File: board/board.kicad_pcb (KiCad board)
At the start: 2 copper layers, 21 x 13 mm, 1 part

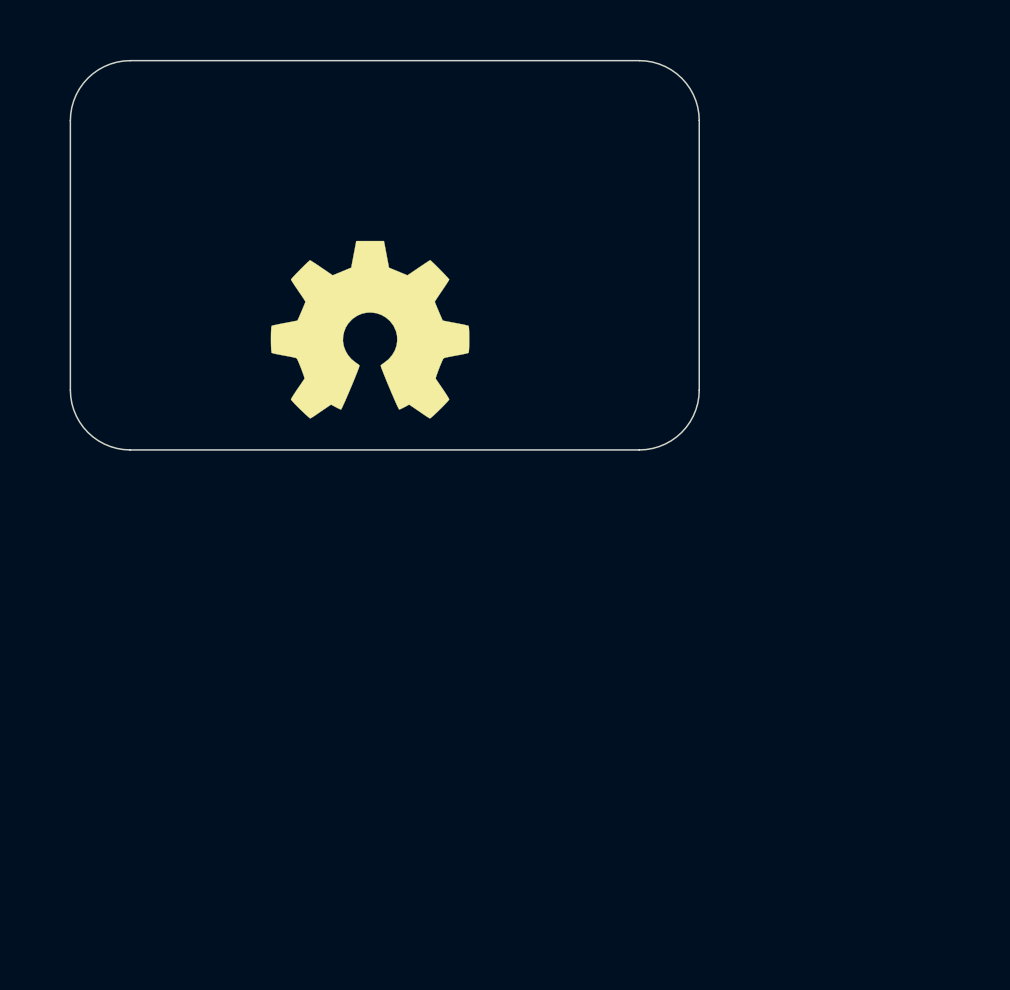
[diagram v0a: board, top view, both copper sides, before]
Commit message: initial
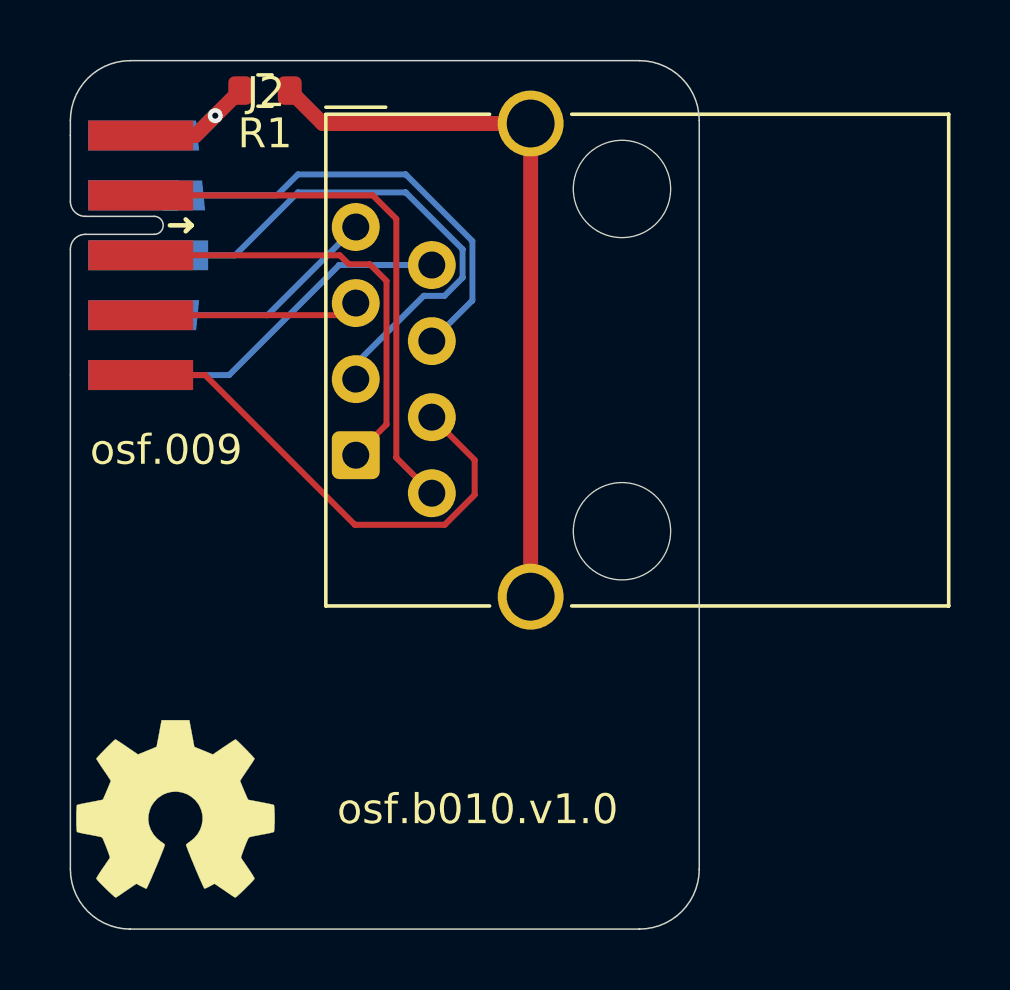
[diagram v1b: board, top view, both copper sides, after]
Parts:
- added J1: 009_1000BASE-T, on_edge:on_edge_2x05_device, F.Cu at (140.0, 96.5)
- added J2: 615008145521, b010:RJ45_Wuerth_615008145521_Horizontal, F.Cu at (149.5, 95.6)
- added R1: 0R, Resistor_SMD:R_0603_1608Metric, F.Cu at (146.5, 91.0)
- moved LOGO1 17.3 mm to (143.5, 115.0)
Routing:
- net /rj45/SCHIELD: track 0.00 -> 24.3 mm
- net /rj45/TD1+: track 0.00 -> 18.5 mm
- net /rj45/TD3-: track 0.00 -> 18.4 mm
- net /rj45/TD2-: track 0.00 -> 16.8 mm
- net /rj45/TD3+: track 0.00 -> 16.4 mm
- net /rj45/TD1-: track 0.00 -> 14.8 mm
- net /rj45/TD4-: track 0.00 -> 11.3 mm
- net /rj45/TD4+: track 0.00 -> 8.35 mm
- net /rj45/TD2+: track 0.00 -> 7.35 mm
- net Earth: track 0.00 -> 6.66 mm, vias 0 -> 1
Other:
- board size 21 x 13 mm -> 21 x 29 mm
- board text added: "osf.009"
- board text added: "osf.b010.v1.0"
